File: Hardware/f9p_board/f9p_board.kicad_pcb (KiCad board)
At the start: 4 copper layers, 75 x 41 mm, 99 parts, among them J1 USB_B_Mini, J10 SERV_3, J2 USB_B_Mini, J3 BAT_CONN, J4 CAN, J5 USB_A_PWR_OUTPUT, J6 EN_BAT_VIN, J7 SERV_0, J8 SERV_1, J9 SERV_2, P1 SWD, Q1 DMN62D0UW-7, SW1 F9P_USB_POWER, SW2 MCU_USB_POWER, SW3 BOOT0, U1 Ublox_ZED_F9P, U2 STM32F405RGTx, U3 MCP16311MS, U4 ncv8705, U5 BMI160, U6 TJA1051TK-3, U7 uFL_conn, U8 TPS54561DPRR, U9 PDS760-13, Y1 8Mhz

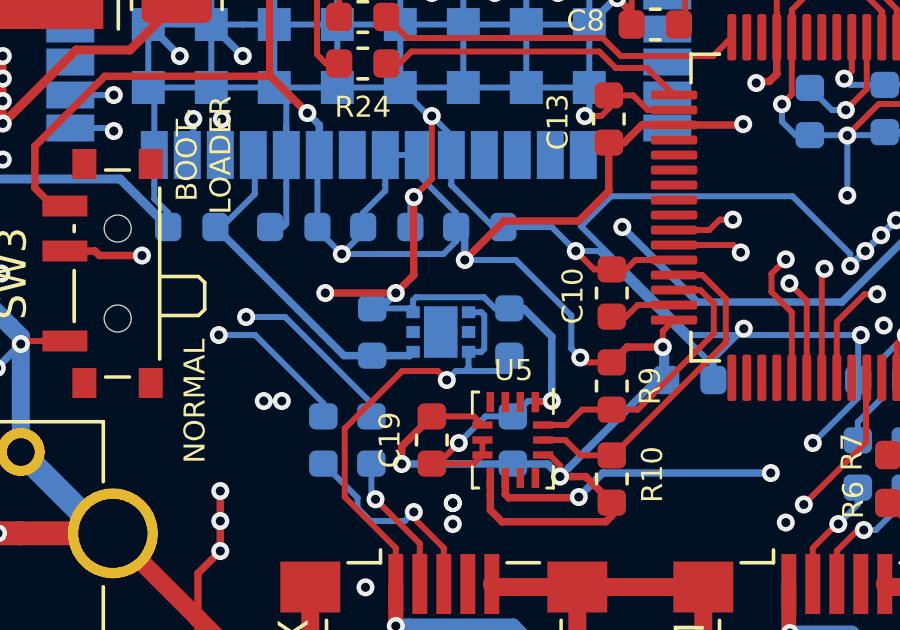
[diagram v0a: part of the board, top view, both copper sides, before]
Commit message: f9p_board added lots of ordernr from digikey and a stp file for rf connector
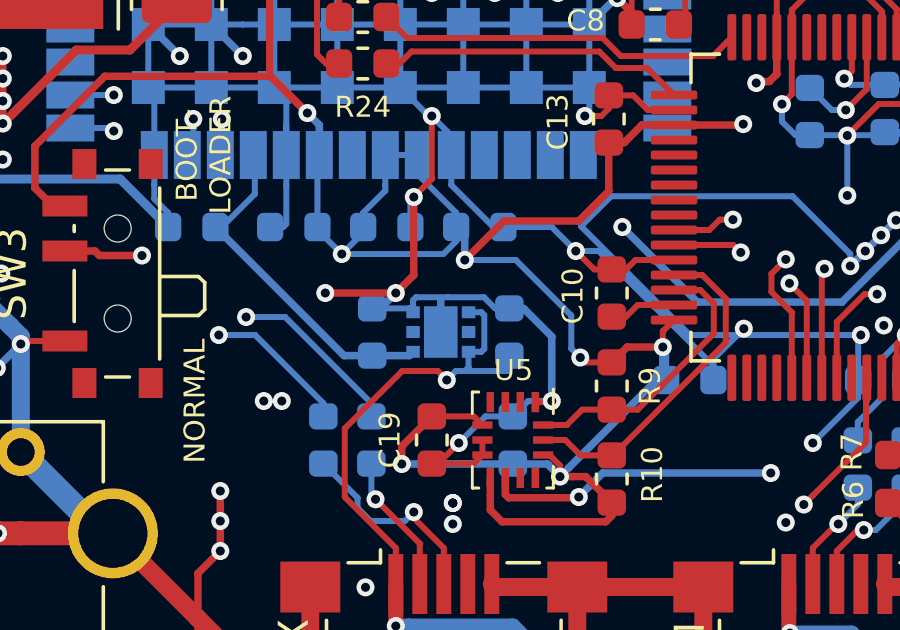
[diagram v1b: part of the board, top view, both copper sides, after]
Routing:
- net GND: track 761.5 -> 762.6 mm
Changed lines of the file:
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@@
-(kicad_pcb (version 20190905) (host pcbnew "5.99.0-unknown-9339afc~100~ubuntu16.04.1")
+(kicad_pcb (version 20190905) (host pcbnew "5.99.0-unknown-a3229c4~86~ubuntu18.04.1")
   (general
     (thickness 1.6)
     (drawings 38)
-    (tracks 1573)
+    (tracks 1575)
     (modules 99)
     (nets 141)
@@
     (effects (font (size 0.7 0.7) (thickness 0.15)) (justify mirror))
   )
+  (segment (start 92.339999 76.539999) (end 91.275001 76.539999) (width 0.2) (layer "B.Cu") (net 5))
+  (segment (start 93.538499 76.539999) (end 92.339999 76.539999) (width 0.2) (layer "B.Cu") (net 5))
+  (segment (start 92.1 76.59) (end 92.1 77.7) (width 0.25) (layer "B.Cu") (net 5))
   (segment (start 83.3 66.7375) (end 81.7375 68.3) (width 0.3) (layer "F.Cu") (net 5))
   (segment (start 81.7375 68.3) (end 79.95 68.3) (width 0.3) (layer "F.Cu") (net 5))
@@
   (segment (start 91.0475 76.9125) (end 91.175 77.04) (width 0.2) (layer "B.Cu") (net 5))
   (segment (start 94.386 76.9125) (end 93.911 76.9125) (width 0.2) (layer "B.Cu") (net 5))
-  (segment (start 93.538499 76.539999) (end 91.275001 76.539999) (width 0.2) (layer "B.Cu") (net 5))
   (segment (start 93.911 76.9125) (end 93.538499 76.539999) (width 0.2) (layer "B.Cu") (net 5))
   (segment (start 91.275001 76.539999) (end 91.175 76.64) (width 0.2) (layer "B.Cu") (net 5))
@@
     (connect_pads yes (clearance 0.3))
     (min_thickness 0.254)
-    (fill yes (thermal_gap 0.508) (thermal_bridge_width 0.508))
+    (fill (thermal_gap 0.508) (thermal_bridge_width 0.508))
     (polygon
       (pts
@@
     (connect_pads (clearance 0.4))
     (min_thickness 0.254)
-    (fill yes (thermal_gap 0.508) (thermal_bridge_width 0.508))
+    (fill (thermal_gap 0.508) (thermal_bridge_width 0.508))
     (polygon
       (pts
@@
     (connect_pads yes (clearance 0.5))
     (min_thickness 0.254)
-    (fill yes (thermal_gap 0.508) (thermal_bridge_width 0.508))
+    (fill (thermal_gap 0.508) (thermal_bridge_width 0.508))
     (polygon
       (pts
@@
     (connect_pads yes (clearance 0.5))
     (min_thickness 0.254)
-    (fill yes (thermal_gap 0.508) (thermal_bridge_width 0.508))
+    (fill (thermal_gap 0.508) (thermal_bridge_width 0.508))
     (polygon
       (pts
@@
     (connect_pads (clearance 0.4))
     (min_thickness 0.254)
-    (fill yes (thermal_gap 0.508) (thermal_bridge_width 0.508))
+    (fill (thermal_gap 0.508) (thermal_bridge_width 0.508))
     (polygon
       (pts
@@
     (connect_pads yes (clearance 0.5))
     (min_thickness 0.254)
-    (fill yes (thermal_gap 0.508) (thermal_bridge_width 0.508))
+    (fill (thermal_gap 0.508) (thermal_bridge_width 0.508))
     (polygon
       (pts
@@
     (connect_pads (clearance 0.4))
     (min_thickness 0.254)
-    (fill yes (thermal_gap 0.508) (thermal_bridge_width 0.508))
+    (fill (thermal_gap 0.508) (thermal_bridge_width 0.508))
     (polygon
       (pts
@@
     (connect_pads (clearance 0.4))
     (min_thickness 0.254)
-    (fill yes (thermal_gap 0.508) (thermal_bridge_width 0.508))
+    (fill (thermal_gap 0.508) (thermal_bridge_width 0.508))
     (polygon
       (pts
@@
     (connect_pads yes (clearance 0.3))
     (min_thickness 0.254)
-    (fill yes (thermal_gap 0.508) (thermal_bridge_width 0.508))
+    (fill (thermal_gap 0.508) (thermal_bridge_width 0.508))
     (polygon
       (pts
